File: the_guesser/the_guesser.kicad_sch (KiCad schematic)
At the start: 2 parts, among them U1 CC1200, U2 ESP32-PICO-D4

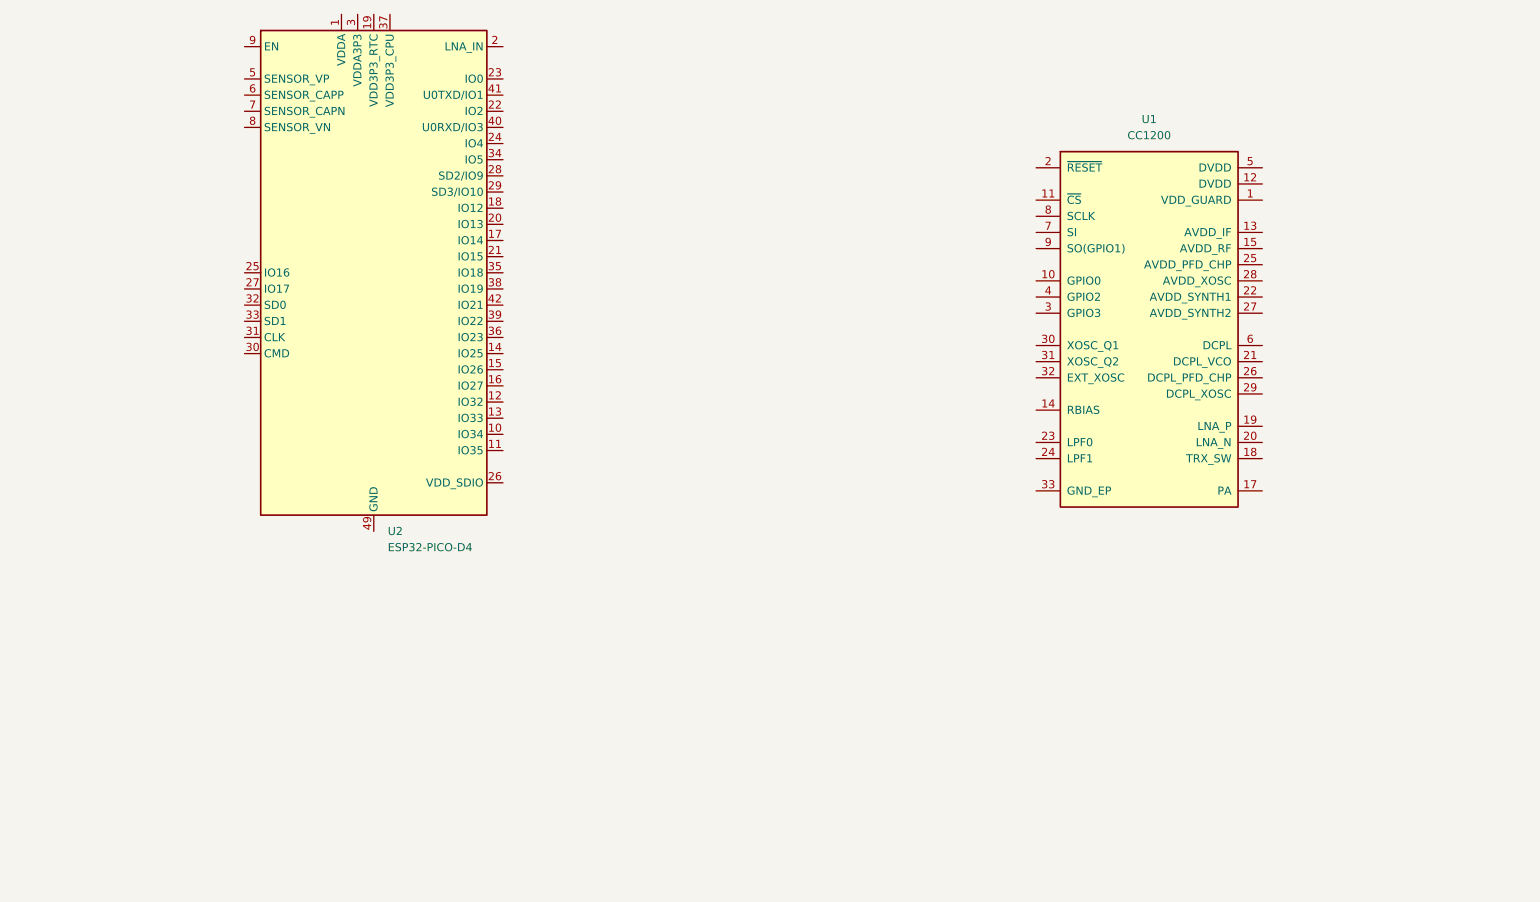
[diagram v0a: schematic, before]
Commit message: created project common symbols library & guesser work
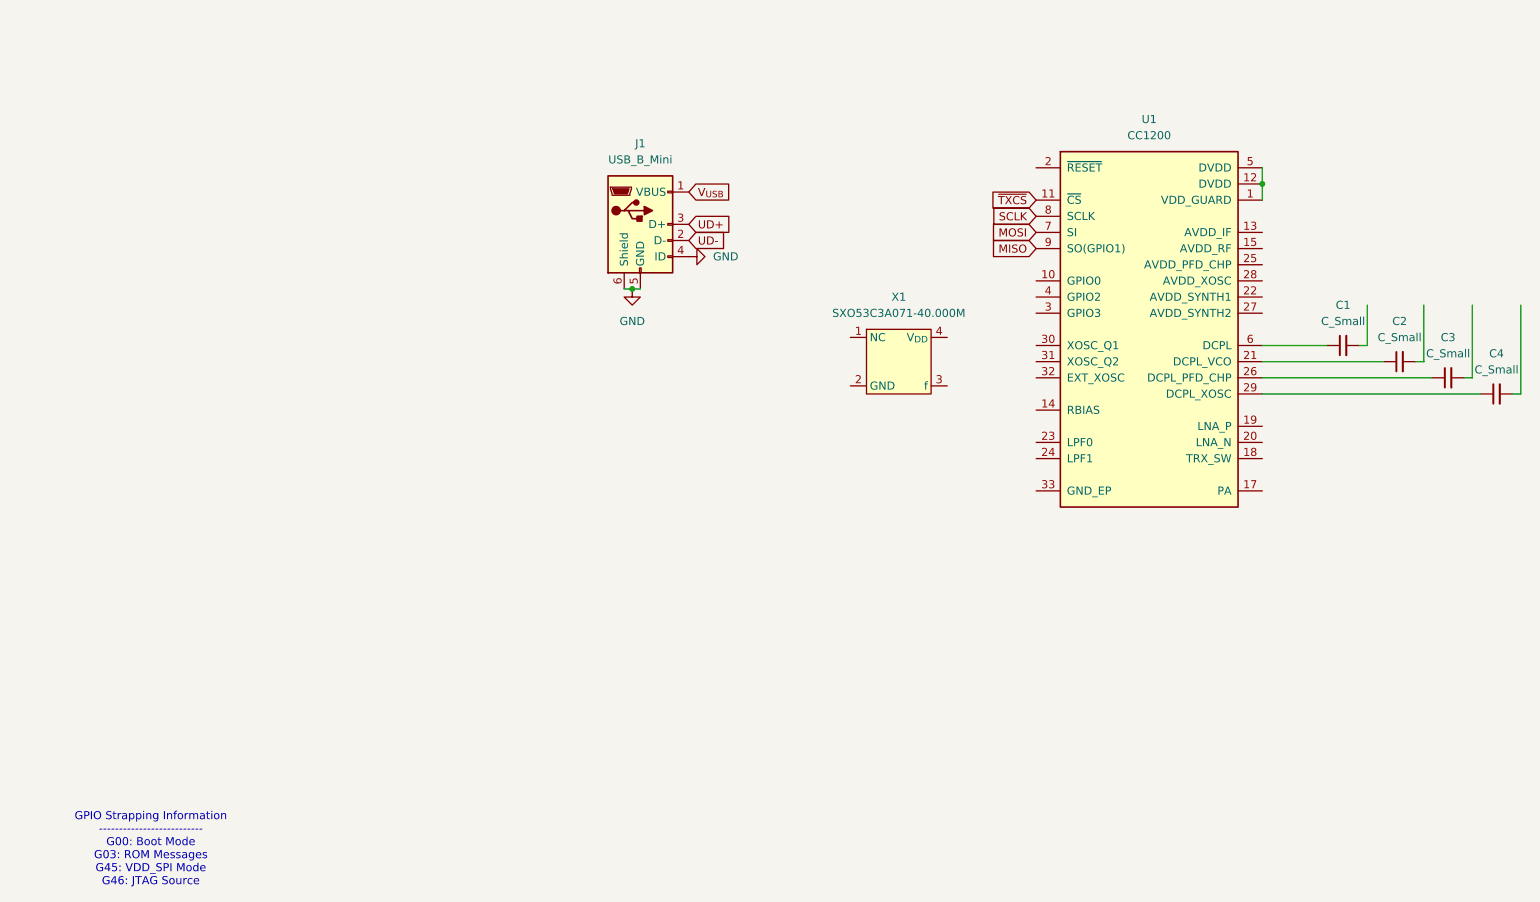
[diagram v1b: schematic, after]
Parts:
- removed U2: ESP32-PICO-D4, Package_DFN_QFN:QFN-48-1EP_7x7mm_P0.5mm_EP5.3x5.3mm, symbol MCU_Espressif:ESP32-PICO-D4
- added C1, C2, C3, C4: C_Small, symbol Device:C_Small
- added J1: USB_B_Mini, symbol Connector:USB_B_Mini
- added X1: SXO53C3A071-40.000M, Crystal:Crystal_SMD_5032-4Pin_5.0x3.2mm, symbol locals:SXO53C3A071-40.000M
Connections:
- net at U1.1 (VDD_GUARD): now also U1.12 (DVDD), U1.5 (DVDD)
- net ~{TXCS}: now reaches U1.11 (~{CS})
- net at U1.21 (DCPL_VCO): now also C2.1
- net at U1.26 (DCPL_PFD_CHP): now also C3.1
- net at U1.29 (DCPL_XOSC): now also C4.1
- net at U1.6 (DCPL): now also C1.1
- net MOSI: now reaches U1.7 (SI)
- net SCLK: now reaches U1.8 (SCLK)
- net MISO: now reaches U1.9 (SO(GPIO1))
- new net GND: J1.4 (ID), J1.5 (GND), J1.6 (Shield)
- new net UD+: J1.3 (D+)
- new net UD-: J1.2 (D-)
- new net V_{USB}: J1.1 (VBUS)
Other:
- note added: "GPIO Strapping Information -------------------------- G00: Boot Mode G03: ROM Messages G45: VDD_SPI Mode G46: JTAG Source"
